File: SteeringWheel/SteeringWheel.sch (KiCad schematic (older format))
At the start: 4 parts, among them J1 Conn_01x02_Male, U1 RC1602A, U2 MCP23008-xP

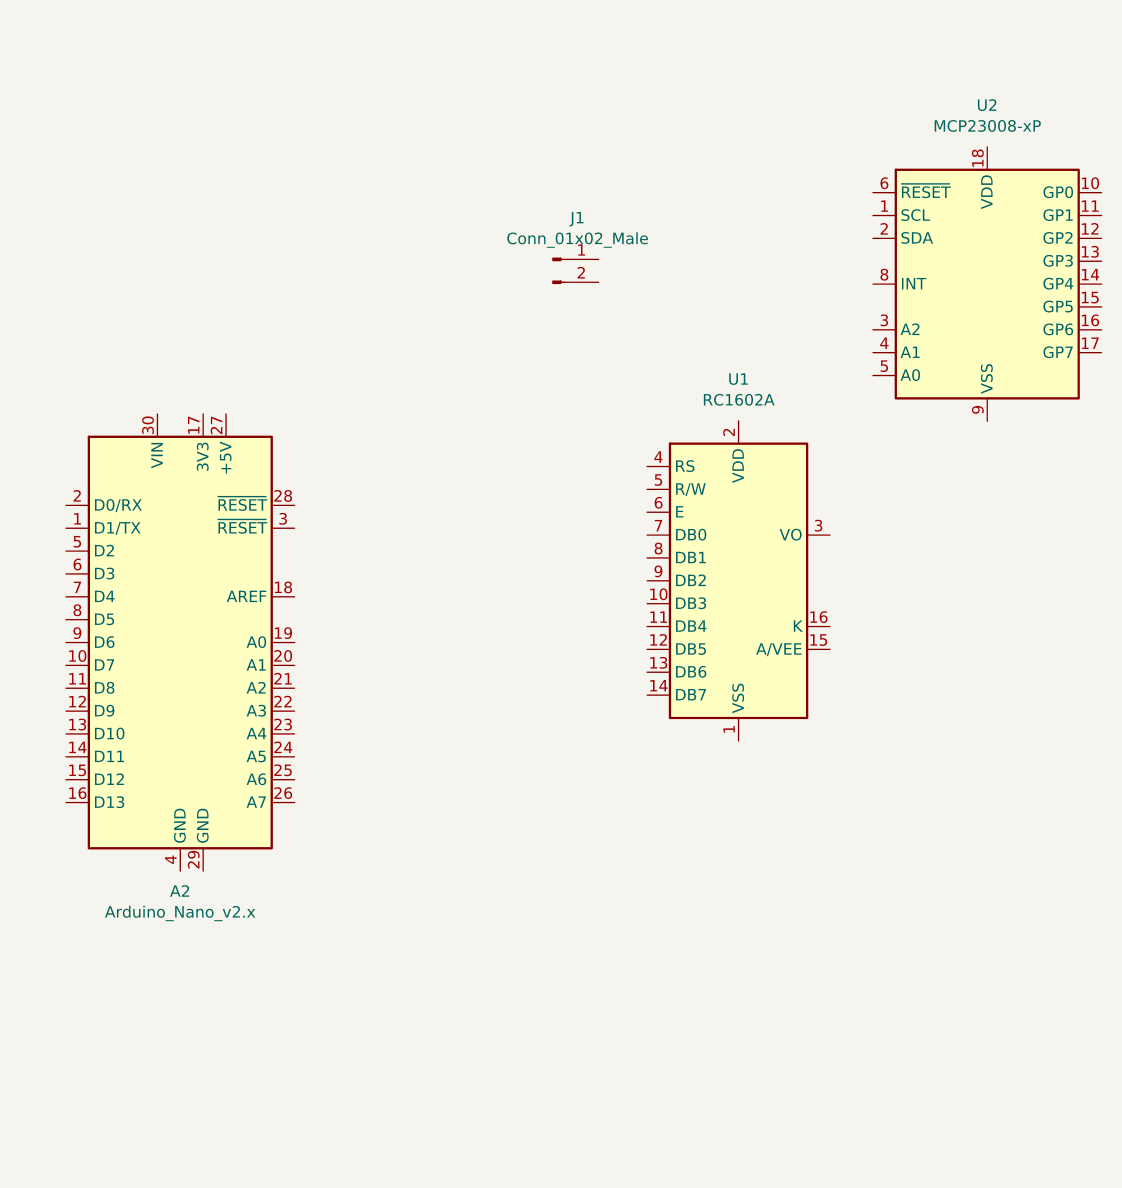
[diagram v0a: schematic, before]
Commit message: Layout
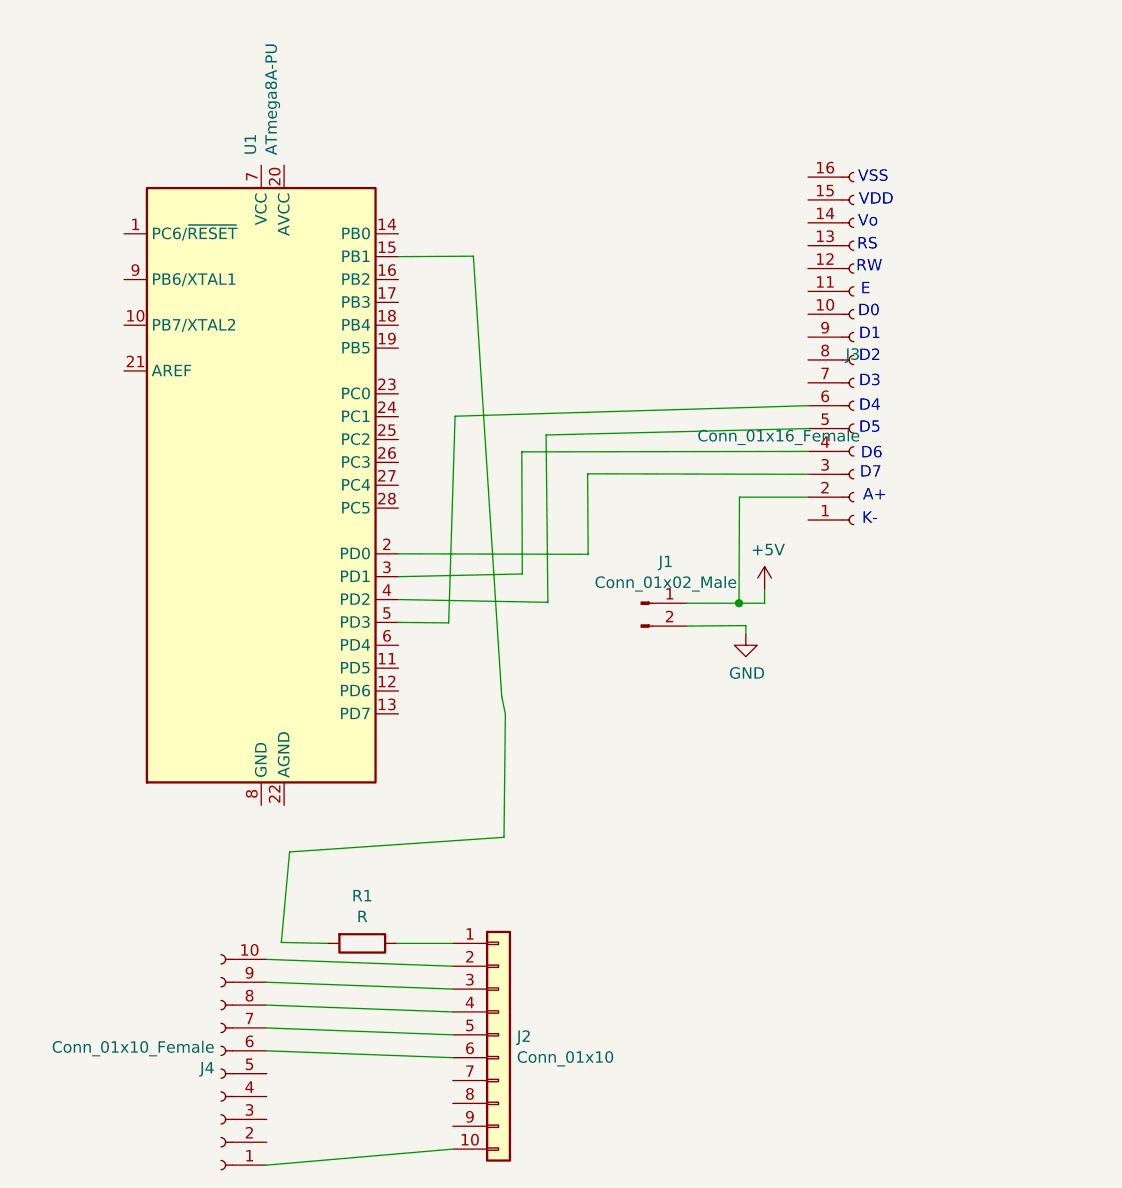
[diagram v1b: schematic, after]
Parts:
- removed A2: Arduino_Nano_v2.x, Module:Arduino_Nano, symbol MCU_Module:Arduino_Nano_v2.x
- removed U1: RC1602A, Display:RC1602A, symbol Display_Character:RC1602A
- removed U2: MCP23008-xP, Package_DIP:DIP-18_W7.62mm, symbol Interface_Expansion:MCP23008-xP
- added J2: Conn_01x10, TerminalBlock_Phoenix:TerminalBlock_Phoenix_MKDS-1,5-10-5.08_1x10_P5.08mm_Horizontal, symbol Connector_Generic:Conn_01x10
- added J3: Conn_01x16_Female, Connector_PinSocket_2.54mm:PinSocket_1x16_P2.54mm_Vertical, symbol Connector:Conn_01x16_Female
- added J4: Conn_01x10_Female, TerminalBlock_Phoenix:TerminalBlock_Phoenix_MKDS-1,5-10-5.08_1x10_P5.08mm_Horizontal, symbol Connector:Conn_01x10_Female
- added R1: R, Resistor_THT:R_Axial_DIN0204_L3.6mm_D1.6mm_P7.62mm_Horizontal, symbol Device:R
- added U1: ATmega8A-PU, Package_DIP:DIP-28_W7.62mm, symbol MCU_Microchip_ATmega:ATmega8A-PU
- J1: footprint TerminalBlock_Phoenix:TerminalBlock_Phoenix_MKDS-1,5-2_1x02_P5.00mm_Horizontal -> TerminalBlock_Phoenix:TerminalBlock_Phoenix_MKDS-1,5-2-5.08_1x02_P5.08mm_Horizontal
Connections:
- net labels added: +5V, GND
- wire segments 0 -> 33
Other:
- note added: "A+\n"
- note added: "D0\n"
- note added: "D1\n"
- note added: "D2\n"
- note added: "D3\n"
- note added: "D4\n"
- note added: "D5\n"
- note added: "D6\n"
- note added: "D7\n"
- note added: "E"
- note added: "K-\n"
- note added: "RS\n"
- note added: "RW\n"
- note added: "VDD"
- note added: "VSS"
- note added: "Vo\n"
- moved on the sheet: J1
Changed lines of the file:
@@
 $EndDescr
 $Comp
-L Display_Character:RC1602A U1
-U 1 1 630ACCFE
-P 5276 3062
-F 0 "U1" H 5276 3943 50  0000 C CNN
-F 1 "RC1602A" H 5276 3852 50  0000 C CNN
-F 2 "Display:RC1602A" H 5376 2262 50  0001 C CNN
-F 3 "http://www.raystar-optronics.com/down.php?ProID=18" H 5376 2962 50  0001 C CNN
-	1    5276 3062
+L Connector:Conn_01x02_Male J1
+U 1 1 630C6641
+P 4850 3160
+F 0 "J1" H 4958 3341 50  0000 C CNN
+F 1 "Conn_01x02_Male" H 4958 3250 50  0000 C CNN
+F 2 "TerminalBlock_Phoenix:TerminalBlock_Phoenix_MKDS-1,5-2-5.08_1x02_P5.08mm_Horizontal" H 4850 3160 50  0001 C CNN
+F 3 "~" H 4850 3160 50  0001 C CNN
+	1    4850 3160
 	1    0    0    -1
 $EndComp
 $Comp
-L Interface_Expansion:MCP23008-xP U2
-U 1 1 630C4E62
-P 6364 1764
-F 0 "U2" H 6364 2545 50  0000 C CNN
-F 1 "MCP23008-xP" H 6364 2454 50  0000 C CNN
-F 2 "Package_DIP:DIP-18_W7.62mm" H 6364 714 50  0001 C CNN
-F 3 "http://ww1.microchip.com/downloads/en/DeviceDoc/MCP23008-MCP23S08-Data-Sheet-20001919F.pdf" H 7664 564 50  0001 C CNN
-	1    6364 1764
+L MCU_Microchip_ATmega:ATmega8A-PU U1
+U 1 1 631447EE
+P 3188 2644
+F 0 "U1" V 3142 4088 50  0000 L CNN
+F 1 "ATmega8A-PU" V 3233 4088 50  0000 L CNN
+F 2 "Package_DIP:DIP-28_W7.62mm" H 3188 2644 50  0001 C CIN
+F 3 "http://ww1.microchip.com/downloads/en/DeviceDoc/Microchip%208bit%20mcu%20AVR%20ATmega8A%20data%20sheet%2040001974A.pdf" H 3188 2644 50  0001 C CNN
+	1    3188 2644
 	1    0    0    -1
 $EndComp
 $Comp
-L MCU_Module:Arduino_Nano_v2.x A2
-U 1 1 630C464E
-P 2834 3332
-F 0 "A2" H 2834 2243 50  0000 C CNN
-F 1 "Arduino_Nano_v2.x" H 2834 2152 50  0000 C CNN
-F 2 "Module:Arduino_Nano" H 2834 3332 50  0001 C CIN
-F 3 "https://www.arduino.cc/en/uploads/Main/ArduinoNanoManual23.pdf" H 2834 3332 50  0001 C CNN
-	1    2834 3332
+L power:+5V #PWR0101
+U 1 1 6314AC6B
+P 5390 3100
+F 0 "#PWR0101" H 5390 2950 50  0001 C CNN
+F 1 "+5V" H 5405 3273 50  0000 C CNN
+F 2 "" H 5390 3100 50  0001 C CNN
+F 3 "" H 5390 3100 50  0001 C CNN
+	1    5390 3100
 	1    0    0    -1
 $EndComp
 $Comp
-L Connector:Conn_01x02_Male J1
-U 1 1 630C6641
-P 4464 1656
-F 0 "J1" H 4572 1837 50  0000 C CNN
-F 1 "Conn_01x02_Male" H 4572 1746 50  0000 C CNN
-F 2 "TerminalBlock_Phoenix:TerminalBlock_Phoenix_MKDS-1,5-2_1x02_P5.00mm_Horizontal" H 4464 1656 50  0001 C CNN
-F 3 "~" H 4464 1656 50  0001 C CNN
-	1    4464 1656
+L power:GND #PWR0102
+U 1 1 6314B9E3
+P 5308 3294
+F 0 "#PWR0102" H 5308 3044 50  0001 C CNN
+F 1 "GND" H 5313 3121 50  0000 C CNN
+F 2 "" H 5308 3294 50  0001 C CNN
+F 3 "" H 5308 3294 50  0001 C CNN
+	1    5308 3294
 	1    0    0    -1
 $EndComp
+Wire Wire Line
+	5390 3160 5390 3100
+Wire Wire Line
+	5308 3258 5050 3260
+Wire Wire Line
+	5308 3258 5308 3294
+Wire Wire Line
+	5278 3160 5280 2696
+Wire Wire Line
+	5280 2696 5580 2696
+$Comp
+L Connector_Generic:Conn_01x10 J2
+U 1 1 63160366
+P 4226 5048
+F 0 "J2" H 4306 5040 50  0000 L CNN
+F 1 "Conn_01x10" H 4306 4949 50  0000 L CNN
+F 2 "TerminalBlock_Phoenix:TerminalBlock_Phoenix_MKDS-1,5-10-5.08_1x10_P5.08mm_Horizontal" H 4226 5048 50  0001 C CNN
+F 3 "~" H 4226 5048 50  0001 C CNN
+	1    4226 5048
+	1    0    0    -1
+$EndComp
+Text Notes 5820 2722 0    50   ~ 0
+A+\n
+Text Notes 5816 2824 0    50   ~ 0
+K-\n
+Text Notes 5806 2622 0    50   ~ 0
+D7\n
+Text Notes 5810 2538 0    50   ~ 0
+D6\n
+Text Notes 5802 2426 0    50   ~ 0
+D5\n
+Text Notes 5802 2330 0    50   ~ 0
+D4\n
+Text Notes 5802 2222 0    50   ~ 0
+D3\n
+$Comp
+L Connector:Conn_01x16_Female J3
+U 1 1 631F38D9
+P 5780 2096
+F 0 "J3" H 5808 2072 50  0000 R CNN
+F 1 "Conn_01x16_Female" H 5808 2429 50  0000 R CNN
+F 2 "Connector_PinSocket_2.54mm:PinSocket_1x16_P2.54mm_Vertical" H 5780 2096 50  0001 C CNN
+F 3 "~" H 5780 2096 50  0001 C CNN
+	1    5780 2096
+	1    0    0    1
+$EndComp
+Text Notes 5802 2112 0    50   ~ 0
+D2\n
+Text Notes 5802 2016 0    50   ~ 0
+D1\n
+Text Notes 5798 1916 0    50   ~ 0
+D0\n
+Text Notes 5810 1820 0    50   ~ 0
+E
+Text Notes 5790 1720 0    50   ~ 0
+RW\n
+Text Notes 5794 1624 0    50   ~ 0
+RS\n
+Text Notes 5798 1524 0    50   ~ 0
+Vo\n
+Text Notes 5802 1428 0    50   ~ 0
+VDD
+Text Notes 5798 1328 0    50   ~ 0
+VSS
+Wire Wire Line
+	5390 3160 5278 3160
+Connection ~ 5278 3160
+Wire Wire Line
+	5278 3160 5050 3160
+$Comp
+L Device:R R1
+U 1 1 6316DF5D
+P 3630 4648
+F 0 "R1" V 3423 4648 50  0000 C CNN
+F 1 "R" V 3514 4648 50  0000 C CNN
+F 2 "Resistor_THT:R_Axial_DIN0204_L3.6mm_D1.6mm_P7.62mm_Horizontal" V 3560 4648 50  0001 C CNN
+F 3 "~" H 3630 4648 50  0001 C CNN
+	1    3630 4648
+	0    1    1    0
+$EndComp
+Wire Wire Line
+	4026 4648 3780 4648
+Wire Wire Line
+	3480 4648 3276 4644
+Wire Wire Line
+	3276 4644 3312 4248
+Wire Wire Line
+	3312 4248 4250 4184
+Wire Wire Line
+	4250 4184 4256 3644
+Wire Wire Line
+	3788 1644 4116 1642
+Wire Wire Line
+	4116 1642 4240 3568
+Wire Wire Line
+	4256 3644 4240 3568
+Wire Wire Line
+	3788 2944 4618 2946
+Wire Wire Line
+	4618 2946 4616 2594
+Wire Wire Line
+	4616 2594 5580 2596
+Wire Wire Line
+	5580 2496 4328 2498
+Wire Wire Line
+	4328 2498 4330 3032
+Wire Wire Line
+	4330 3032 3788 3044
+Wire Wire Line
+	3788 3144 4442 3156
+Wire Wire Line
+	4442 3156 4434 2424
+Wire Wire Line
+	4434 2424 5580 2396
+Wire Wire Line
+	5580 2296 4036 2342
+Wire Wire Line
+	4036 2342 4008 3246
+Wire Wire Line
+	4008 3246 3788 3244
+$Comp
+L Connector:Conn_01x10_Female J4
+U 1 1 63152CD3
+P 3012 5218
+F 0 "J4" H 3040 5194 50  0000 L CNN
+F 1 "Conn_01x10_Female" H 3040 5103 50  0000 L CNN
+F 2 "TerminalBlock_Phoenix:TerminalBlock_Phoenix_MKDS-1,5-10-5.08_1x10_P5.08mm_Horizontal" H 3012 5218 50  0001 C CNN
+F 3 "~" H 3012 5218 50  0001 C CNN
+	1    3012 5218
+	-1   0    0    1
+$EndComp
+Wire Wire Line
+	4026 4748 3212 4718
+Wire Wire Line
+	3212 4818 4026 4848
+Wire Wire Line
+	4026 4948 3212 4918
+Wire Wire Line
+	4024 5048 3212 5018
+Wire Wire Line
+	4026 5148 3212 5118
+Wire Wire Line
+	3212 5618 4026 5548
 $EndSCHEMATC

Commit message: update
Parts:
- J2, J4: footprint TerminalBlock_Phoenix:TerminalBlock_Phoenix_MKDS-1,5-10-5.08_1x10_P5.08mm_Horizontal -> TerminalBlock_Phoenix:TerminalBlock_Phoenix_MPT-0,5-10-2.54_1x10_P2.54mm_Horizontal
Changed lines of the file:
@@
 F 0 "J2" H 4306 5040 50  0000 L CNN
 F 1 "Conn_01x10" H 4306 4949 50  0000 L CNN
-F 2 "TerminalBlock_Phoenix:TerminalBlock_Phoenix_MKDS-1,5-10-5.08_1x10_P5.08mm_Horizontal" H 4226 5048 50  0001 C CNN
+F 2 "TerminalBlock_Phoenix:TerminalBlock_Phoenix_MPT-0,5-10-2.54_1x10_P2.54mm_Horizontal" H 4226 5048 50  0001 C CNN
 F 3 "~" H 4226 5048 50  0001 C CNN
 	1    4226 5048
@@
 F 0 "J4" H 3040 5194 50  0000 L CNN
 F 1 "Conn_01x10_Female" H 3040 5103 50  0000 L CNN
-F 2 "TerminalBlock_Phoenix:TerminalBlock_Phoenix_MKDS-1,5-10-5.08_1x10_P5.08mm_Horizontal" H 3012 5218 50  0001 C CNN
+F 2 "TerminalBlock_Phoenix:TerminalBlock_Phoenix_MPT-0,5-10-2.54_1x10_P2.54mm_Horizontal" H 3012 5218 50  0001 C CNN
 F 3 "~" H 3012 5218 50  0001 C CNN
 	1    3012 5218
